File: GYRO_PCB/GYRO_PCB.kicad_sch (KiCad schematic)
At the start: 4 parts, among them J1 Pmod GYRO, J2 FLASH Socket 1, J3 FLASH Socket 2, U1 NUCLEO-F446RE

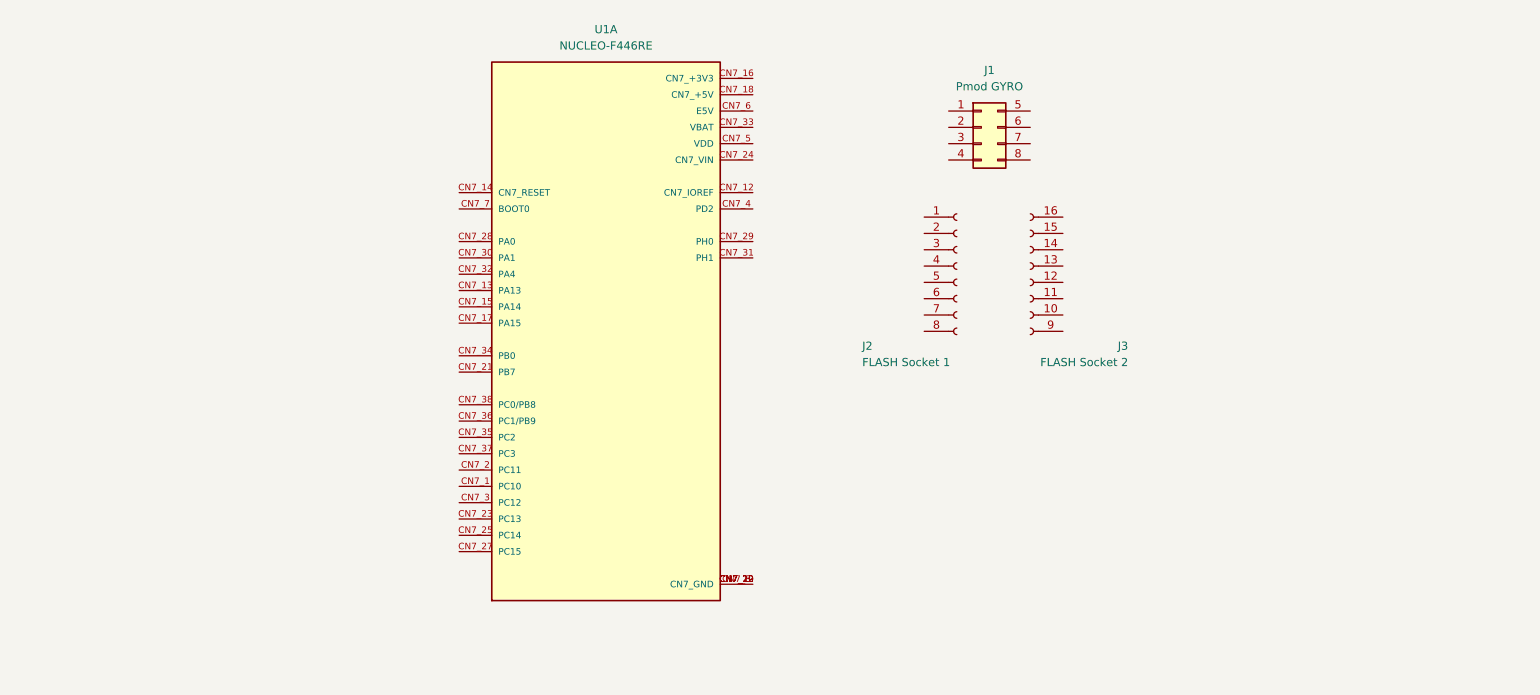
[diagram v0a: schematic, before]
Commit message: feat: most of schematic done
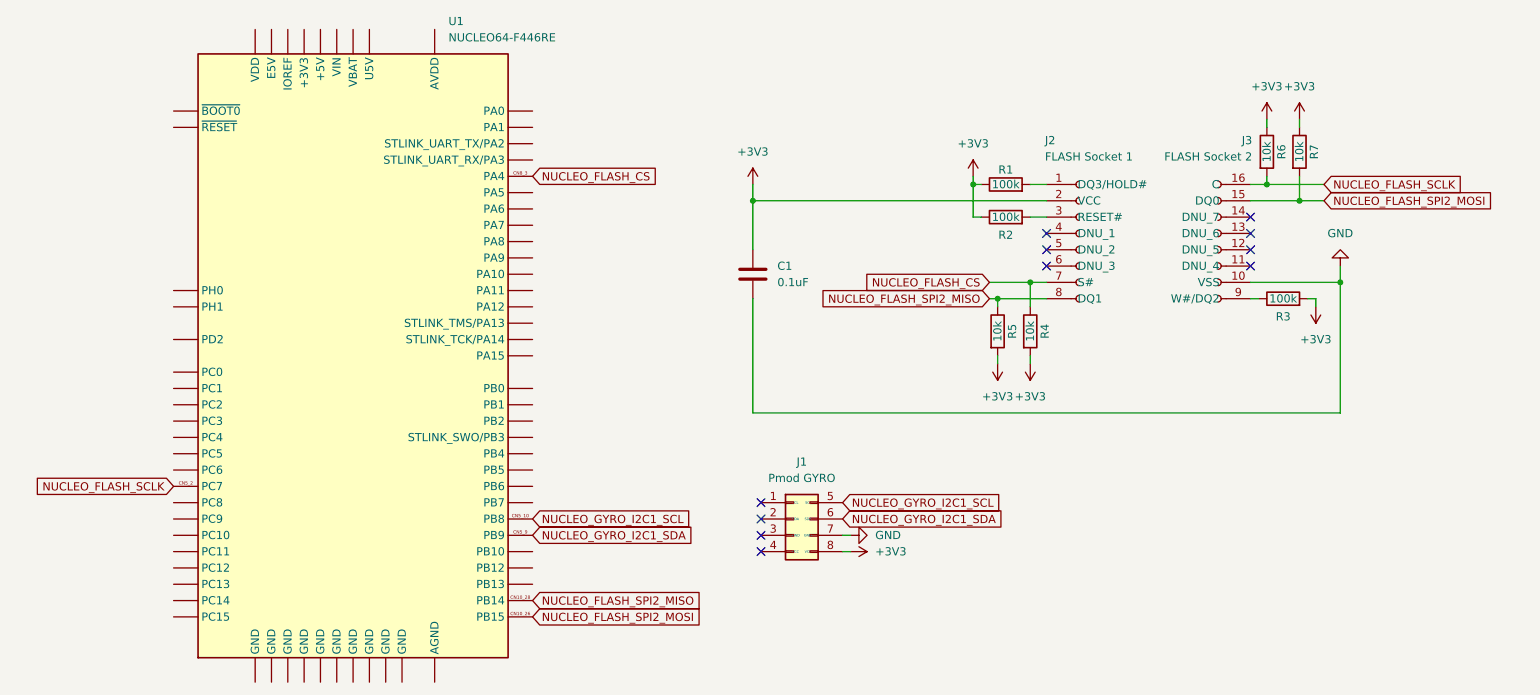
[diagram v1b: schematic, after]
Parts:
- removed U1: NUCLEO-F446RE, FOOTPRINTS:NUCLEO-F446RE, symbol NUCLEO-F446RE:NUCLEO-F446RE
- added C1: 0.1uF, symbol Device:C
- added R1, R2, R3: 100k, symbol Device:R
- added R4, R5, R6, R7: 10k, symbol Device:R
- added U1: NUCLEO64-F446RE, FOOTPRINTS:NUCLEO-F446RE, symbol NUCLEO-F446RE:NUCLEO64-F411RE
- J1: footprint Connector_PinSocket_2.54mm:PinSocket_2x04_P2.54mm_Vertical -> GYRO:PinSocket_2x04_P2.54mm_Vertical_Custom
- J3: footprint Connector_PinSocket_2.54mm:PinSocket_1x08_P2.54mm_Vertical -> GYRO:PinSocket_1x08_P2.54mm_Vertical_Custom
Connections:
- net GND: now reaches J3.10 (VSS)
- net GND: now also J1.7 (GND), C1.2
- net NUCLEO_FLASH_SPI2_MOSI: now reaches J3.15 (DQ0)
- net NUCLEO_FLASH_SPI2_MOSI: now also R7.2, U1.CN10_26 (PB15)
- net NUCLEO_FLASH_SCLK: now reaches J3.16 (C)
- net NUCLEO_FLASH_SCLK: now also R6.2, U1.CN5_2 (PC7)
- net at J3.9 (W#/DQ2): now also R3.1
- net at J2.1 (DQ3/HOLD#): now also R1.2
- net +3V3: now reaches J2.2 (VCC)
- net +3V3: now also J1.8 (VCC), C1.1, R1.1, R2.1, R3.2, R4.2, R5.2, R6.1, R7.1
- net at J2.3 (RESET#): now also R2.2
- net NUCLEO_FLASH_CS: now reaches J2.7 (S#)
- net NUCLEO_FLASH_CS: now also R4.1, U1.CN8_3 (PA4)
- net NUCLEO_FLASH_SPI2_MISO: now reaches J2.8 (DQ1)
- net NUCLEO_FLASH_SPI2_MISO: now also R5.1, U1.CN10_28 (PB14)
- net NUCLEO_GYRO_I2C1_SCL: now reaches J1.5 (SCL)
- net NUCLEO_GYRO_I2C1_SCL: now also U1.CN5_10 (PB8)
- net NUCLEO_GYRO_I2C1_SDA: now reaches J1.6 (SDA)
- net NUCLEO_GYRO_I2C1_SDA: now also U1.CN5_9 (PB9)
- no-connect marks 0 -> 11
